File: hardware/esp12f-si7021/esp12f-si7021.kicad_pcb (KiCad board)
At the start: 2 copper layers, 36.8 x 63.5 mm, 17 parts, among them J1 Battery, J2 UART, U1 TPS613221ADBV, U2 ESP-12F, U3 Si7021-A20

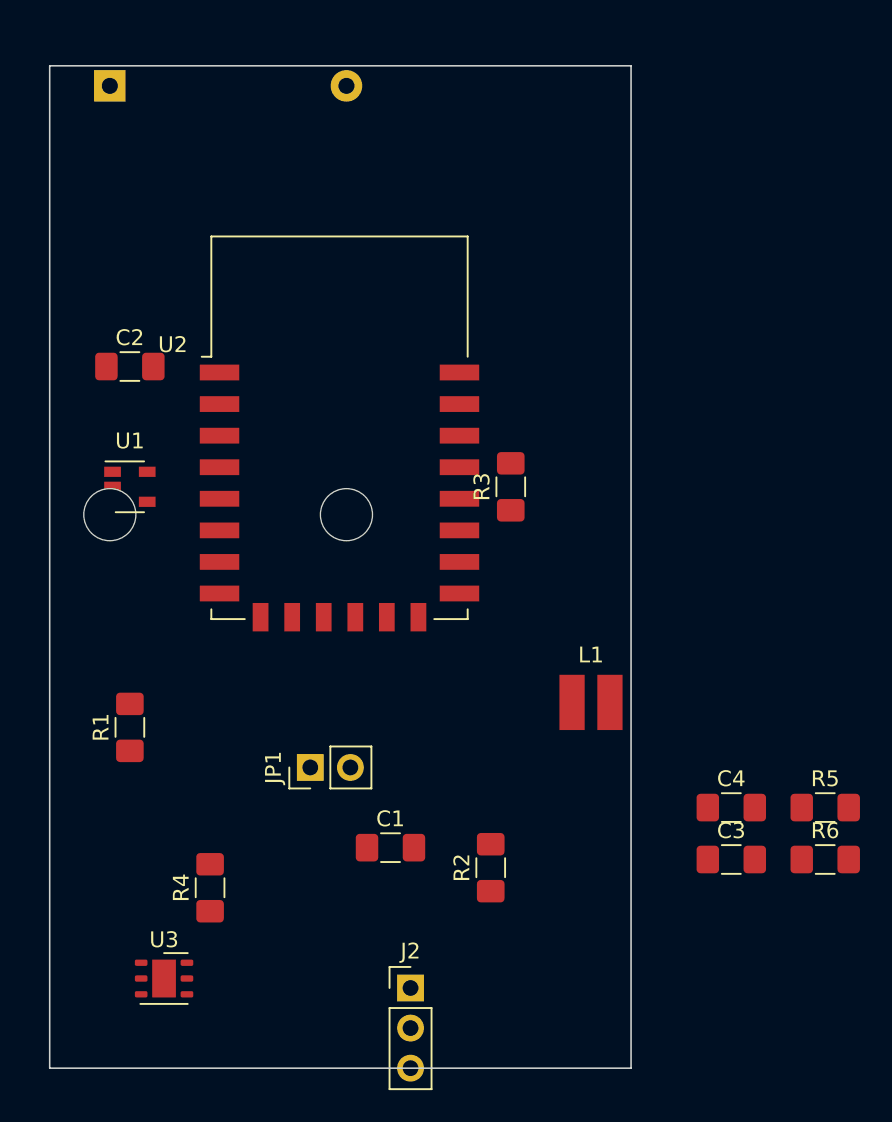
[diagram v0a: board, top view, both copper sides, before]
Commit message: Update to v1.1
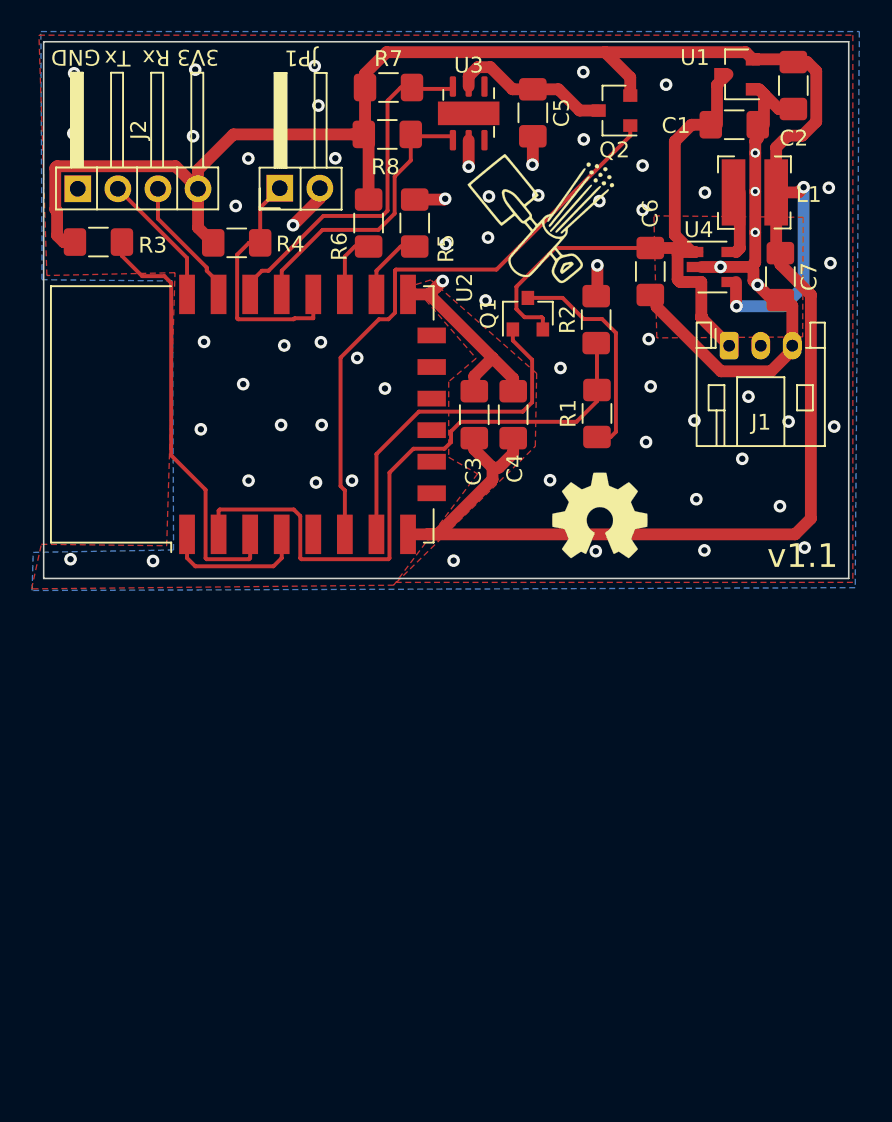
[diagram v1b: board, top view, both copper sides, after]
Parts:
- added C5: 0.1uF, Capacitor_SMD:C_1206_3216Metric_Pad1.42x1.75mm_HandSolder, F.Cu at (44.6, 18.2)
- added C6: 4.7uF, Capacitor_SMD:C_1206_3216Metric_Pad1.42x1.75mm_HandSolder, F.Cu at (52.0, 28.3)
- added C7: 10uF, Capacitor_SMD:C_1206_3216Metric_Pad1.42x1.75mm_HandSolder, F.Cu at (60.3, 28.6)
- added G***: LOGO, kicad-custom:ganthorpe-fibre, F.Cu at (45.4, 24.8)
- added G***: LOGO, kicad-custom:open-hardware, F.Cu at (48.8, 43.7)
- added Q1: BSS84, Package_TO_SOT_SMD:SOT-23, F.Cu at (44.3, 30.9)
- added Q2: BSS84, Package_TO_SOT_SMD:SOT-23, F.Cu at (49.7, 18.1)
- added R7: 10K, Resistor_SMD:R_1206_3216Metric_Pad1.42x1.75mm_HandSolder, F.Cu at (35.4, 16.6)
- added R8: 10K, Resistor_SMD:R_1206_3216Metric_Pad1.42x1.75mm_HandSolder, F.Cu at (35.4, 19.6)
- added U4: TPS62203, Package_TO_SOT_SMD:SOT-23-5, F.Cu at (56.0, 28.0)
- C1: value 22uF -> 1uF
- C2: value 0.1uF -> 1uF
- C3: value 10uF -> 0.1uF
- C4: value 0.1uF -> 10uF
- J1: footprint Battery:BatteryHolder_Keystone_2462_2xAA -> Connector_JST:JST_PH_S3B-PH-K_1x03_P2.00mm_Horizontal; moved to F.Cu
- J2: footprint Connector_PinHeader_2.54mm:PinHeader_1x03_P2.54mm_Vertical -> Connector_PinHeader_2.54mm:PinHeader_1x04_P2.54mm_Horizontal
- JP1: footprint Connector_PinHeader_2.54mm:PinHeader_1x02_P2.54mm_Vertical -> Connector_PinHeader_2.54mm:PinHeader_1x02_P2.54mm_Horizontal
- L1: value 4.7uH -> 10uH; footprint Inductor_SMD:Multicomp_0302 -> kicad-custom:L_Bourns-SRN4012
- R1: value 10K -> 330K; footprint Capacitor_SMD:C_1206_3216Metric_Pad1.42x1.75mm_HandSolder -> Resistor_SMD:R_1206_3216Metric_Pad1.42x1.75mm_HandSolder
- R2: value 10K -> 100K; footprint Capacitor_SMD:C_1206_3216Metric_Pad1.42x1.75mm_HandSolder -> Resistor_SMD:R_1206_3216Metric_Pad1.42x1.75mm_HandSolder
- R3, R4, R5, R6: footprint Capacitor_SMD:C_1206_3216Metric_Pad1.42x1.75mm_HandSolder -> Resistor_SMD:R_1206_3216Metric_Pad1.42x1.75mm_HandSolder
- U1: value TPS613221ADBV -> MCP1700; footprint Package_TO_SOT_SMD:SOT-23-5 -> Package_TO_SOT_SMD:SOT-23
- U3: value Si7021-A20 -> Si7021
- moved U3 58.1 mm to (40.5, 18.3), turned to 90 degrees
- moved J2 54.8 mm to (15.7, 23.0), turned to 90 degrees
- moved C1 50.7 mm to (57.3, 19.0)
- moved R6 48.0 mm to (37.1, 25.2), turned to 90 degrees
- moved R5 47.0 mm to (34.2, 25.2), turned to 270 degrees
- moved U1 46.5 mm to (57.5, 15.8), turned to 180 degrees
- moved C2 45.6 mm to (61.1, 16.5), turned to 270 degrees
- moved J1 42.5 mm to (57.0, 33.0), turned to 0 degrees
- moved R4 40.9 mm to (25.8, 26.5), turned to 0 degrees
- moved JP1 36.7 mm to (28.5, 23.0)
- moved R1 35.7 mm to (48.6, 37.3)
- moved R2 35.4 mm to (48.6, 31.3)
- moved C3 32.5 mm to (40.9, 37.3), turned to 90 degrees
- moved L1 30.9 mm to (58.8, 23.0)
- moved R3 30.4 mm to (17.1, 26.4), turned to 0 degrees
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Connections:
- C1 pad 1: Net-(C1-Pad1) -> +BATT
- C2 pad 1: Net-(C1-Pad1) -> +3V3
- C3 pad 1: Net-(C1-Pad1) -> +3V3
- C4 pad 1: Net-(C4-Pad1) -> +3V3
- J1 pad 1: Net-(J1-Pad1) -> +BATT
- J1 pad 2: GND -> (no net)
- J2 pad 3: Net-(J2-Pad3) -> /Rx
- L1 pad 1: Net-(J1-Pad1) -> Net-(L1-Pad1)
- L1 pad 2: Net-(L1-Pad2) -> +3V3
- R1 pad 1: Net-(C1-Pad1) -> Net-(Q1-Pad3)
- R2 pad 1: Net-(C1-Pad1) -> Net-(R1-Pad2)
- R2 pad 2: Net-(JP1-Pad1) -> GND
- R3 pad 1: Net-(C1-Pad1) -> +3V3
- R4 pad 1: Net-(R4-Pad1) -> +3V3
- R4 pad 2: GND -> Net-(JP1-Pad1)
- R5 pad 1: Net-(C1-Pad1) -> +3V3
- R6 pad 1: Net-(C1-Pad1) -> Net-(R6-Pad1)
- R6 pad 2: Net-(R6-Pad2) -> GND
- U1 pad 1: Net-(L1-Pad2) -> GND
- U1 pad 2: GND -> +3V3
- U1 pad 3: (no net) -> +BATT
- U2 pad 16: Net-(R4-Pad1) -> Net-(R6-Pad1)
- U2 pad 17: Net-(R3-Pad2) -> Net-(R5-Pad2)
- U2 pad 19: Net-(R6-Pad2) -> Net-(R8-Pad2)
- U2 pad 2: (no net) -> Net-(R1-Pad2)
- U2 pad 20: Net-(R5-Pad2) -> Net-(R7-Pad2)
- U2 pad 21: Net-(J2-Pad2) -> /Rx
- U2 pad 22: Net-(J2-Pad3) -> Net-(J2-Pad2)
- U2 pad 3: Net-(R1-Pad2) -> Net-(R3-Pad2)
- U2 pad 6: (no net) -> Net-(Q2-Pad1)
- U2 pad 7: Net-(C4-Pad1) -> Net-(Q1-Pad1)
- U2 pad 8: Net-(C1-Pad1) -> +3V3
- U3 pad 1: Net-(R6-Pad2) -> Net-(R8-Pad2)
- U3 pad 5: Net-(C4-Pad1) -> Net-(C5-Pad1)
- U3 pad 6: Net-(R5-Pad2) -> Net-(R7-Pad2)
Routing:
- net +3V3: track 0.00 -> 155.9 mm, vias 0 -> 2
- net GND: track 0.00 -> 60.8 mm, vias 0 -> 65
- net +BATT: track 0.00 -> 39.9 mm
- net Net-(R1-Pad2): track 0.00 -> 39.8 mm
- net Net-(Q2-Pad1): track 0.00 -> 37.7 mm
- net Net-(R3-Pad2): track 0.00 -> 27.4 mm
- net Net-(R7-Pad2): track 0.00 -> 22.9 mm
- net Net-(Q1-Pad1): track 0.00 -> 21.4 mm
- net Net-(R8-Pad2): track 0.00 -> 18.3 mm
- net Net-(JP1-Pad1): track 0.00 -> 16.4 mm
- net Net-(Q1-Pad3): track 0.00 -> 14.1 mm
- net Net-(C5-Pad1): track 0.00 -> 9.96 mm
- net Net-(U2-Pad1): track 0.00 -> 9.43 mm
- net Net-(J2-Pad2): track 0.00 -> 8.51 mm
- net /Rx: track 0.00 -> 8.29 mm
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- added copper zone on B.Cu, net GND
- added copper zone on F.Cu, net GND
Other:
- board size 36.8 x 63.5 mm -> 51 x 34 mm
- net class Power added: clearance 0.2, trace_width 0.75, via_dia 0.8, via_drill 0.4
- rule trace_min: 0.2 -> 0.127
- rule via_min_size: 0.4 -> 0.45
- board text added: "3V3"
- board text added: "GND"
- board text added: "JLCJLCJLCJLC"
- board text added: "Rx"
- board text added: "Tx"
- board text added: "v1.1"
